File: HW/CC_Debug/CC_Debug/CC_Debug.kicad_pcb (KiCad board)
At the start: 2 copper layers, 46 parts, among them J3001 USB_B, U2001 USB2514B/M2, U2002 24Mhz,50ppm, U5001 12Mhz,50ppm, U5002 FT4232H_QFN

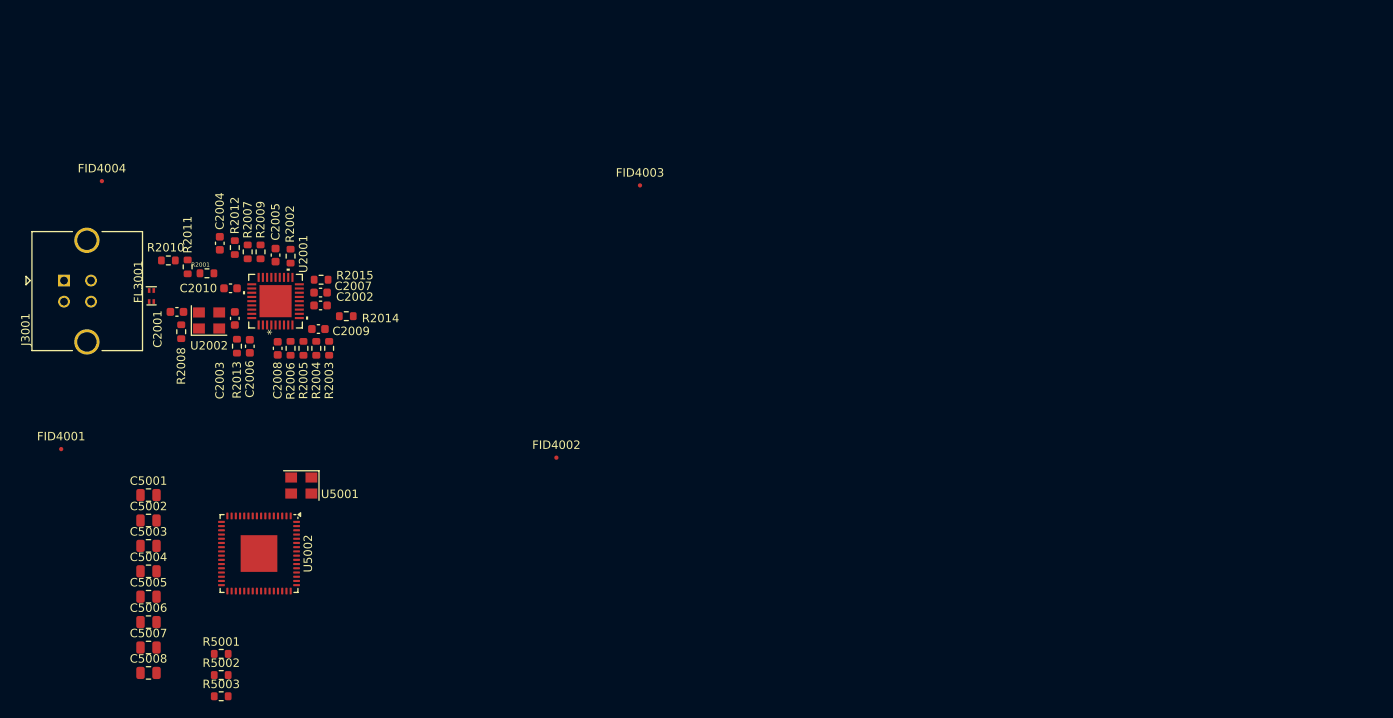
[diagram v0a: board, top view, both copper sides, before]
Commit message: .
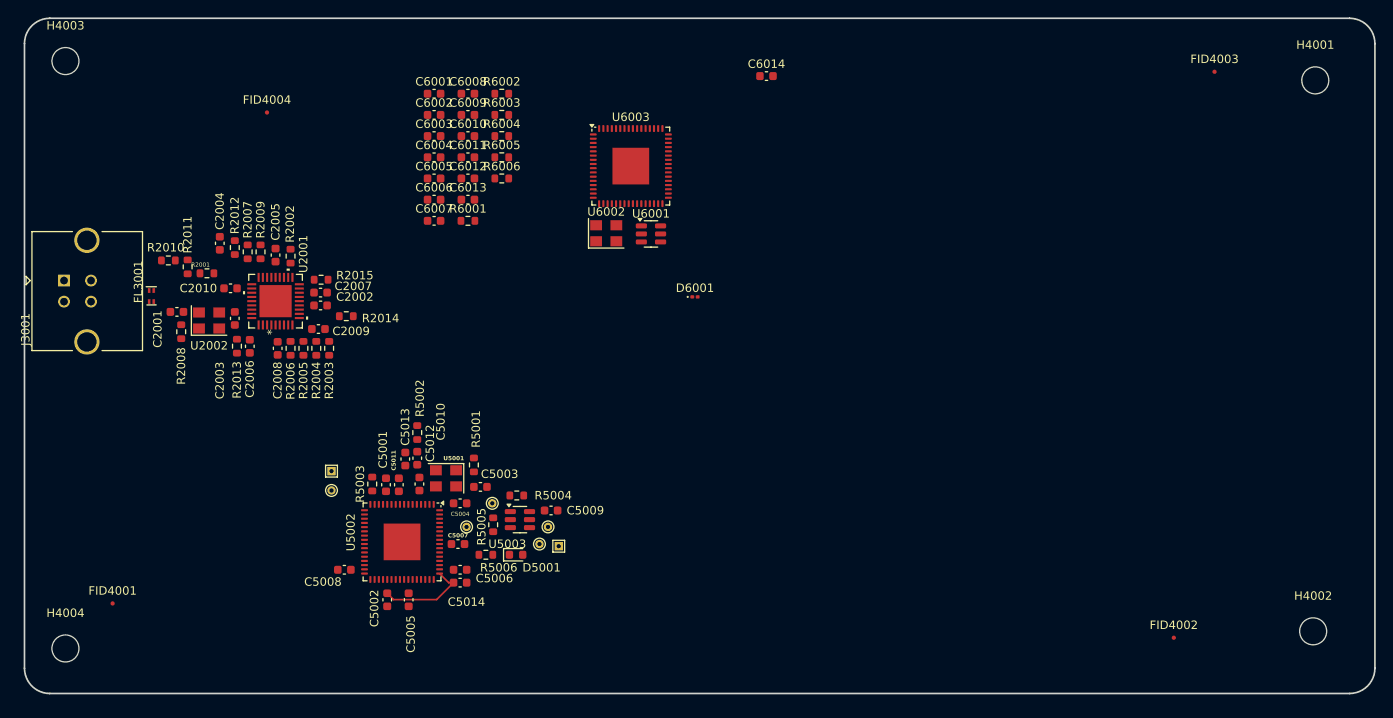
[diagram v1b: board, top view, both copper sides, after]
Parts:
- added C5009: 100n 25V, Capacitor_SMD:C_0603_1608Metric, F.Cu at (148.7, 120.8)
- added C5010: 10u 10V, Capacitor_SMD:C_0603_1608Metric, F.Cu at (132.9, 114.6)
- added C5011: 100n 25V, Capacitor_SMD:C_0603_1608Metric, F.Cu at (130.7, 117.8)
- added C5012: 100n 25V, Capacitor_SMD:C_0603_1608Metric, F.Cu at (133.1, 117.7)
- added C5013: 10u 10V, Capacitor_SMD:C_0603_1608Metric, F.Cu at (131.4, 114.7)
- added C5014: 10u 10V, Capacitor_SMD:C_0603_1608Metric, F.Cu at (137.9, 129.4)
- added C6001: 100n 25V, Capacitor_SMD:C_0603_1608Metric, F.Cu at (134.9, 71.4)
- added C6002: 100n 25V, Capacitor_SMD:C_0603_1608Metric, F.Cu at (134.9, 73.9)
- added C6003: 100n 25V, Capacitor_SMD:C_0603_1608Metric, F.Cu at (134.9, 76.5)
- added C6004: 100n 25V, Capacitor_SMD:C_0603_1608Metric, F.Cu at (134.9, 79.0)
- added C6005: 100n 25V, Capacitor_SMD:C_0603_1608Metric, F.Cu at (134.9, 81.5)
- added C6006: 10u 10V, Capacitor_SMD:C_0603_1608Metric, F.Cu at (134.9, 84.0)
- added C6007: 100n 25V, Capacitor_SMD:C_0603_1608Metric, F.Cu at (134.9, 86.5)
- added C6008: 100n 25V, Capacitor_SMD:C_0603_1608Metric, F.Cu at (138.9, 71.4)
- added C6009: 10u 10V, Capacitor_SMD:C_0603_1608Metric, F.Cu at (138.9, 73.9)
- added C6010: 100n 25V, Capacitor_SMD:C_0603_1608Metric, F.Cu at (138.9, 76.5)
- added C6011: 100n 25V, Capacitor_SMD:C_0603_1608Metric, F.Cu at (138.9, 79.0)
- added C6012: 100n 25V, Capacitor_SMD:C_0603_1608Metric, F.Cu at (138.9, 81.5)
- added C6013: 100n 25V, Capacitor_SMD:C_0603_1608Metric, F.Cu at (138.9, 84.0)
- added C6014: 10u 10V, Capacitor_SMD:C_0603_1608Metric, F.Cu at (174.2, 69.3)
- added D5001: LED, LED_SMD:LED_0603_1608Metric, F.Cu at (144.6, 126.1)
- added D6001: LED, LED_SMD:LED_0201_0603Metric, F.Cu at (165.8, 95.5)
- added H4001: MountingHole, MountingHole:MountingHole_3.2mm_M3, F.Cu at (239.3, 69.8)
- added H4002: MountingHole, MountingHole:MountingHole_3.2mm_M3, F.Cu at (239.0, 135.1)
- added H4003: MountingHole, MountingHole:MountingHole_3.2mm_M3, F.Cu at (91.2, 67.6)
- added H4004: MountingHole, MountingHole:MountingHole_3.2mm_M3, F.Cu at (91.2, 137.2)
- added R5004: 10K, Resistor_SMD:R_0603_1608Metric, F.Cu at (144.7, 119.0)
- added R5005: 2K2, Resistor_SMD:R_0603_1608Metric, F.Cu at (141.9, 122.5)
- added R5006: 510R, Resistor_SMD:R_0603_1608Metric, F.Cu at (141.0, 126.1)
- added R6001: 10K, Resistor_SMD:R_0603_1608Metric, F.Cu at (138.9, 86.5)
- added R6002: 10K, Resistor_SMD:R_0603_1608Metric, F.Cu at (142.9, 71.4)
- added R6003: 2K2, Resistor_SMD:R_0603_1608Metric, F.Cu at (142.9, 73.9)
- added R6004: 12K, Resistor_SMD:R_0603_1608Metric, F.Cu at (142.9, 76.5)
- added R6005: 10K, Resistor_SMD:R_0603_1608Metric, F.Cu at (142.9, 79.0)
- added R6006: 510R, Resistor_SMD:R_0603_1608Metric, F.Cu at (142.9, 81.5)
- added TP5001: TestPoint, TestPoint:TestPoint_THTPad_D1.0mm_Drill0.5mm, F.Cu at (148.4, 122.8)
- added TP5002: TestPoint, TestPoint:TestPoint_THTPad_D1.0mm_Drill0.5mm, F.Cu at (141.8, 120.0)
- added TP5003: TestPoint, TestPoint:TestPoint_THTPad_1.0x1.0mm_Drill0.5mm, F.Cu at (149.6, 125.0)
- added TP5004: TestPoint, TestPoint:TestPoint_THTPad_D1.0mm_Drill0.5mm, F.Cu at (147.3, 124.8)
- added TP5005: TestPoint, TestPoint:TestPoint_THTPad_D1.0mm_Drill0.5mm, F.Cu at (138.7, 122.8)
- added TP5006: TestPoint, TestPoint:TestPoint_THTPad_1.0x1.0mm_Drill0.5mm, F.Cu at (122.7, 116.2)
- added TP5007: TestPoint, TestPoint:TestPoint_THTPad_D1.0mm_Drill0.5mm, F.Cu at (122.7, 118.4)
- added U5003: 93AA46BT-I/OT, Package_TO_SOT_SMD:SOT-23-6, F.Cu at (145.0, 121.9)
- added U6001: 93AA46BT-I/OT, Package_TO_SOT_SMD:SOT-23-6, F.Cu at (160.6, 88.0)
- added U6002: 12Mhz,50ppm, Oscillator:Oscillator_SMD_SeikoEpson_SG8002CE-4Pin_3.2x2.5mm, F.Cu at (155.3, 88.0)
- added U6003: FT4232H_QFN, Package_DFN_QFN:QFN-64-1EP_9x9mm_P0.5mm_EP4.35x4.35mm, F.Cu at (158.2, 80.0)
- C5001, C5002, C5003, C5004, C5005, C5006, C5007, C5008: footprint Capacitor_SMD:C_0805_2012Metric -> Capacitor_SMD:C_0603_1608Metric
- moved FID4002 76.2 mm to (222.5, 135.9)
- moved FID4003 69.4 mm to (227.3, 68.8)
- moved C5003 39.9 mm to (140.4, 118.0)
- moved C5007 38.7 mm to (137.7, 124.8)
- moved C5004 37.8 mm to (137.9, 120.0)
- moved C5006 37.4 mm to (137.9, 127.8)
- moved R5001 37.4 mm to (139.6, 115.4), turned to 90 degrees
- moved R5002 36.9 mm to (132.9, 111.6), turned to 90 degrees
- moved R5003 30.9 mm to (127.5, 117.7), turned to 90 degrees
- moved C5005 30.8 mm to (131.9, 131.4), turned to -90 degrees
- moved C5002 29.8 mm to (129.3, 131.4), turned to -90 degrees
- moved C5001 28.2 mm to (129.2, 117.8), turned to 90 degrees
- moved C5008 26.2 mm to (124.2, 127.8), turned to 180 degrees
- moved FID4004 21.2 mm to (115.1, 73.7)
- moved FID4001 19.3 mm to (96.8, 131.8)
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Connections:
- net Net-(U5001-OUT) renamed /USB2UART1/12Mhz
- net Net-(U5002-REF) renamed /USB2UART1/REF
- net Net-(U5002-~{RESET}) renamed /USB2UART1/RESET#
- U2001 pad 3: /USB hub/USB2.D- -> /USB2.D-
- U2001 pad 4: /USB hub/USB2.D+ -> /USB2.D+
- U5002 pad 16: unconnected-(U5002-ADBUS0-Pad16) -> /USB2UART1/UART_A_1.TX
- U5002 pad 17: unconnected-(U5002-ADBUS1-Pad17) -> /USB2UART1/UART_A_1.RX
- U5002 pad 26: unconnected-(U5002-BDBUS0-Pad26) -> /USB2UART1/UART_A_1.TX
- U5002 pad 27: unconnected-(U5002-BDBUS1-Pad27) -> /USB2UART1/UART_A_2.RX
- U5002 pad 38: unconnected-(U5002-CDBUS0-Pad38) -> /USB2UART1/UART_A_1.TX
- U5002 pad 39: unconnected-(U5002-CDBUS1-Pad39) -> /USB2UART1/UART_A_3.RX
- U5002 pad 48: unconnected-(U5002-DDBUS0-Pad48) -> /USB2UART1/UART_A_4.TX
- U5002 pad 52: unconnected-(U5002-DDBUS1-Pad52) -> /USB2UART1/UART_A_4.RX
- U5002 pad 60: unconnected-(U5002-~{PWREN}-Pad60) -> Net-(U5002-~{PWREN})
- U5002 pad 61: unconnected-(U5002-EEDATA-Pad61) -> /USB2UART1/EEDATA
- U5002 pad 62: unconnected-(U5002-EECLK-Pad62) -> /USB2UART1/EECLK
- U5002 pad 63: unconnected-(U5002-EECS-Pad63) -> /USB2UART1/EECS
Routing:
- net +1V8A: track 0.00 -> 11.1 mm
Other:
- board outline added: 160 x 80 mm
- copper layers 2 -> 4
